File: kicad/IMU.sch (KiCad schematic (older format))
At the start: 3 parts, among them U6 ICM-20602

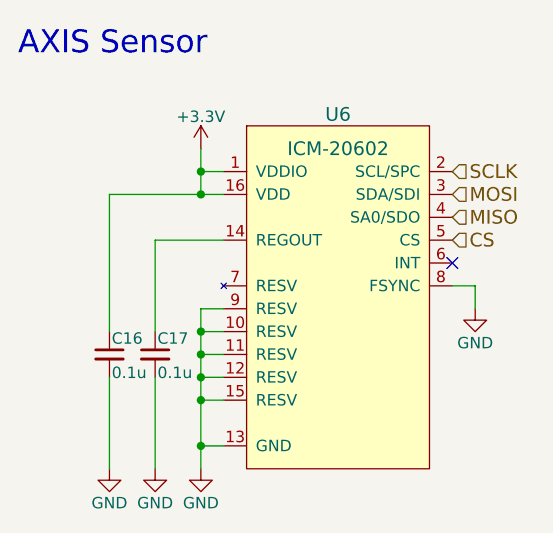
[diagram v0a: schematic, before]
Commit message: アンテナを外側に配置
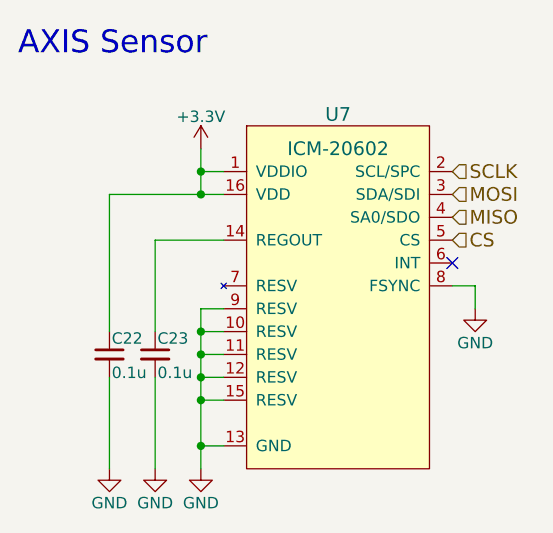
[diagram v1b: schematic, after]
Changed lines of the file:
@@
 AR Path="/57CC33F6/592C611A" Ref="U6"  Part="1"
 AR Path="/5A18D4D6/592C611A" Ref="U7"  Part="1"
-F 0 "U6" H 5600 4150 60  0000 C CNN
+F 0 "U7" H 5600 4150 60  0000 C CNN
 F 1 "ICM-20602" H 5600 4000 60  0000 C CNN
 F 2 "mouse:ICM-20602" H 5600 4000 60  0001 C CNN
@@
 AR Path="/57CC33F6/592C613A" Ref="C17"  Part="1"
 AR Path="/5A18D4D6/592C613A" Ref="C23"  Part="1"
-F 0 "C17" H 4810 3770 50  0000 L CNN
+F 0 "C23" H 4810 3770 50  0000 L CNN
 F 1 "0.1u" H 4810 3620 50  0000 L CNN
 F 2 "Capacitor_SMD:C_0201_0603Metric" H 4800 3700 50  0001 C CNN
@@
 AR Path="/57CC33F6/592C6186" Ref="C16"  Part="1"
 AR Path="/5A18D4D6/592C6186" Ref="C22"  Part="1"
-F 0 "C16" H 4610 3770 50  0000 L CNN
+F 0 "C22" H 4610 3770 50  0000 L CNN
 F 1 "0.1u" H 4610 3620 50  0000 L CNN
 F 2 "Capacitor_SMD:C_0201_0603Metric" H 4600 3700 50  0001 C CNN

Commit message: フットプリントを改良
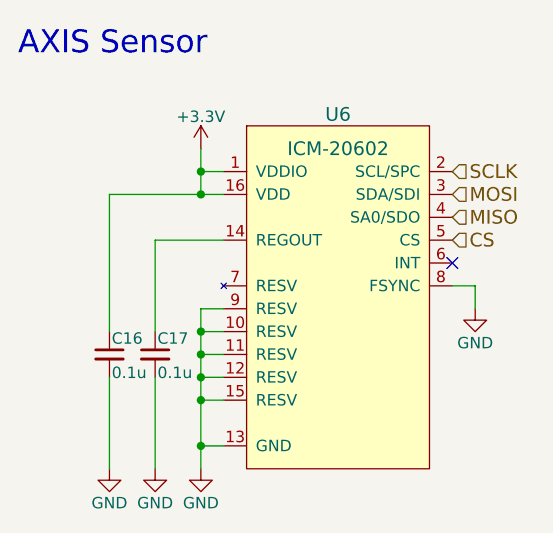
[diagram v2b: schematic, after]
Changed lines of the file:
@@
 AR Path="/57CC33F6/592C611A" Ref="U6"  Part="1"
 AR Path="/5A18D4D6/592C611A" Ref="U7"  Part="1"
-F 0 "U7" H 5600 4150 60  0000 C CNN
+F 0 "U6" H 5600 4150 60  0000 C CNN
 F 1 "ICM-20602" H 5600 4000 60  0000 C CNN
 F 2 "mouse:ICM-20602" H 5600 4000 60  0001 C CNN
@@
 AR Path="/57CC33F6/592C613A" Ref="C17"  Part="1"
 AR Path="/5A18D4D6/592C613A" Ref="C23"  Part="1"
-F 0 "C23" H 4810 3770 50  0000 L CNN
+F 0 "C17" H 4810 3770 50  0000 L CNN
 F 1 "0.1u" H 4810 3620 50  0000 L CNN
 F 2 "Capacitor_SMD:C_0201_0603Metric" H 4800 3700 50  0001 C CNN
@@
 AR Path="/57CC33F6/592C6186" Ref="C16"  Part="1"
 AR Path="/5A18D4D6/592C6186" Ref="C22"  Part="1"
-F 0 "C22" H 4610 3770 50  0000 L CNN
+F 0 "C16" H 4610 3770 50  0000 L CNN
 F 1 "0.1u" H 4610 3620 50  0000 L CNN
 F 2 "Capacitor_SMD:C_0201_0603Metric" H 4600 3700 50  0001 C CNN
